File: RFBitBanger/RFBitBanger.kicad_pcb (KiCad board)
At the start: 2 copper layers, 152 x 88 mm, 226 parts, among them J1 POWER, J10 si5351mod, J11 SPEAKER, J12 Conn_Coaxial, J13 Conn_01x01, J14 Conn_01x01, J15 Conn_01x01, J16 Conn_01x01, J17 Filt1, J18 Filt2, J19 Conn_01x20, J2 Barrel_Jack, J20 Conn_01x01, J21 Conn_01x01, J3 Conn_01x01, J4 Conn_01x01, J5 Conn_01x04, J6 Conn_01x01, J7 Conn_01x01, J8 Conn_01x01, J9 ICSP, P1 Mini-DIN_6pins_ver4, Q1 2N3904, Q10 2N3904, Q11 2N3904, Q12 2N3904, Q13 SS8050, Q14 2N3904, Q15 NC, Q2 2N3904, Q3 2N7000, Q4 2N3904, Q5 NC, Q6 2N7000, Q7 2N7000, Q8 SS8050, Q9 2N7000, SW1 SW_Push, SW2 SW_Push, SW3 SW_Push, SW4 SW_Push, SW5 SW_Push, SW6 SW_Push, T1 Trifilar, T2 Trifilar, T3 Current, T4 Common-Mode Choke, U1 ATMEGA328-PU, U2 LM7805_TO220, U3 LM386, U4 LM358, U5 LCD1602ExtraPins, U6 SI5351A, Y1 16 MHz, Y2 7.X MHz, Y3 27 MHz, Y4 7.X MHz, Y5 7.X MHz

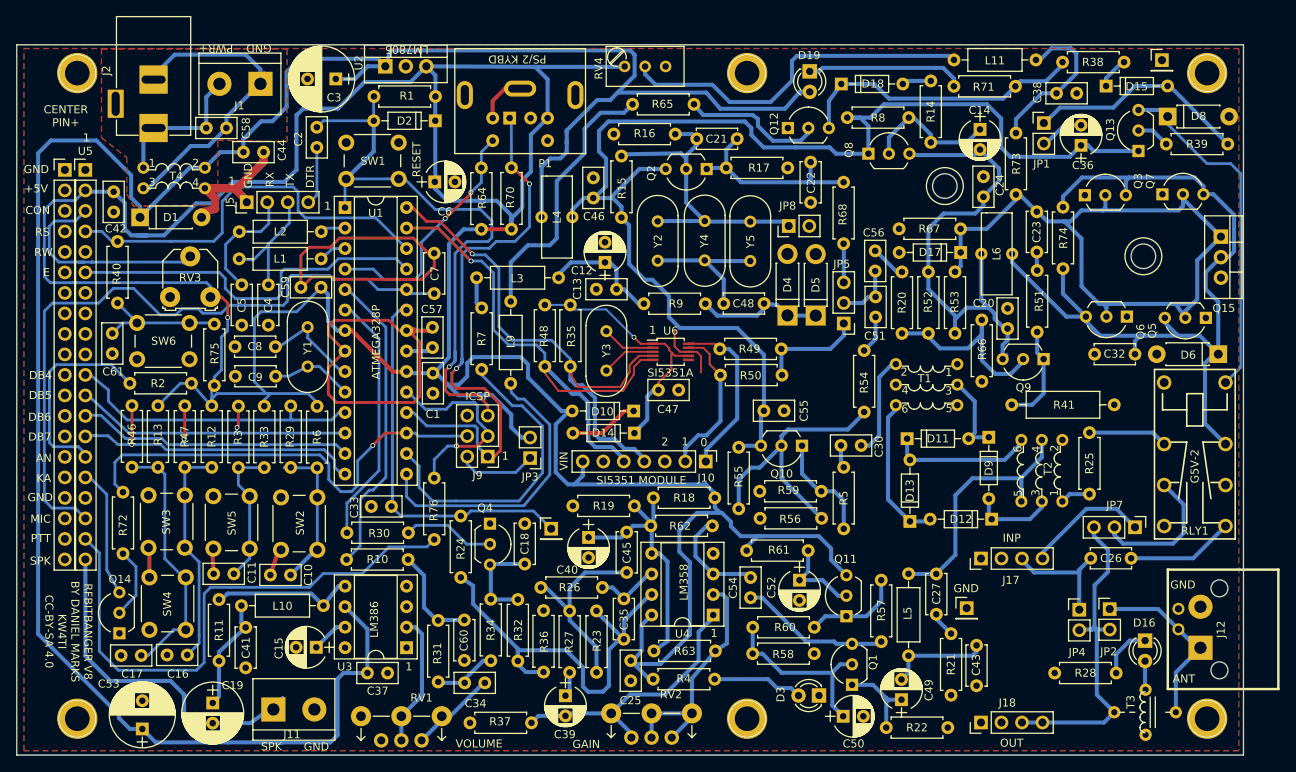
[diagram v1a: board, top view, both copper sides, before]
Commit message: Converted all Kicad projects to version 6.0.10
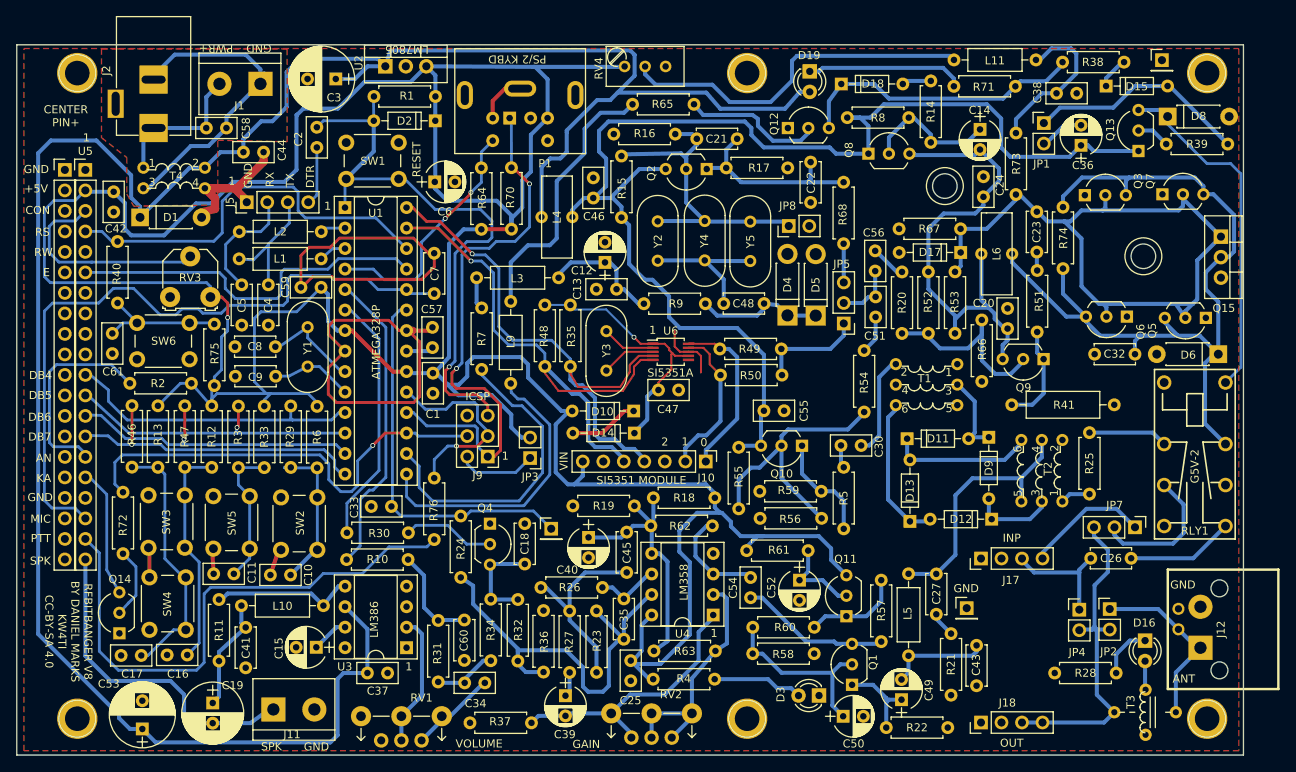
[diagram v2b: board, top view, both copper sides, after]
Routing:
- net +5V: track 421.3 -> 415.6 mm
- net Net-(C36-Pad1): track 162.0 -> 158.1 mm
- net AMPOUT: track 109.2 -> 105.7 mm
- net Net-(C14-Pad2): track 63.7 -> 60.5 mm
- net Net-(C23-Pad2): track 91.5 -> 89.2 mm
- net MICPADDLE: track 87.6 -> 85.2 mm
- net +12V: track 279.1 -> 276.8 mm
- net Net-(C19-Pad1): track 16.8 -> 14.8 mm
- net RESET: track 77.5 -> 75.9 mm
- net TXRELAY: track 44.8 -> 43.2 mm
- net SPKR: track 46.3 -> 45.0 mm
- net Net-(C50-Pad1): track 24.3 -> 23.0 mm
- net TUNING: track 40.4 -> 39.1 mm
- net Net-(C14-Pad1): track 18.6 -> 17.3 mm
- net Net-(C16-Pad2): track 29.1 -> 27.9 mm
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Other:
- net class Default removed

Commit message: Added RFBitBangerNano
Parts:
- C48: value 100 nF -> 100 pF
- Q13, Q8: value SS8050 -> SS8550
- R49, R50: value 100R -> 47R
- R73: value 1k -> 10k
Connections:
- J10 pad 3: (no net) -> unconnected-(J10-Pad3)
- J2 pad 3: (no net) -> unconnected-(J2-Pad3)
- RLY1 pad 3: (no net) -> Net-(RLY1-Pad3)
- RLY1 pad 8: (no net) -> unconnected-(RLY1-Pad8)
- U3 pad 1: (no net) -> unconnected-(U3-Pad1)
- U3 pad 8: (no net) -> unconnected-(U3-Pad8)
- U5 pad 10: (no net) -> unconnected-(U5-Pad10)
- U5 pad 7: (no net) -> unconnected-(U5-Pad7)
- U5 pad 8: (no net) -> unconnected-(U5-Pad8)
- U5 pad 9: (no net) -> unconnected-(U5-Pad9)
- U6 pad 6: (no net) -> unconnected-(U6-Pad6)
